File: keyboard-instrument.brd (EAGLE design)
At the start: 68.6 x 53.3 mm, 9 parts

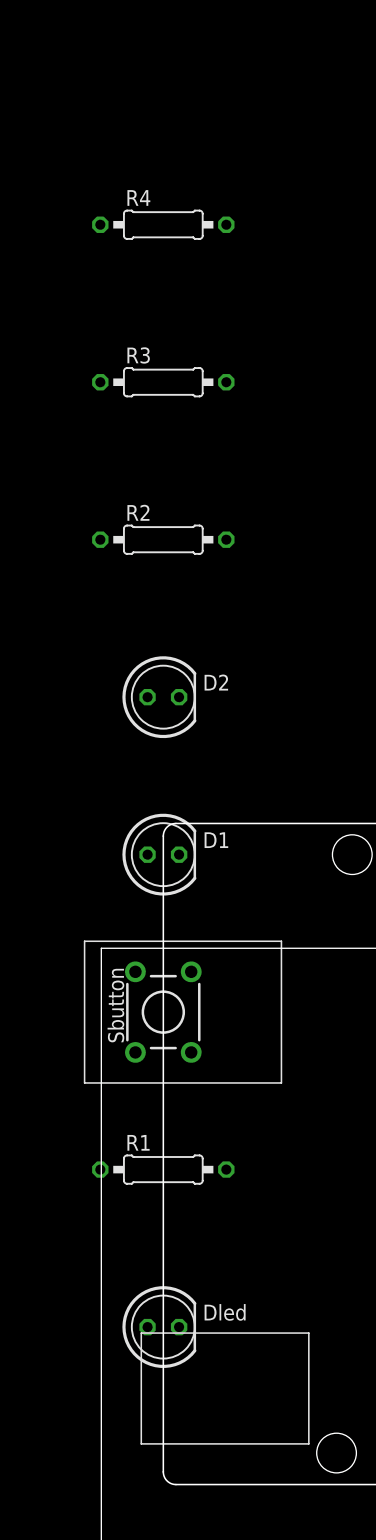
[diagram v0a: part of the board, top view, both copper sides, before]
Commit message: Added code and brd
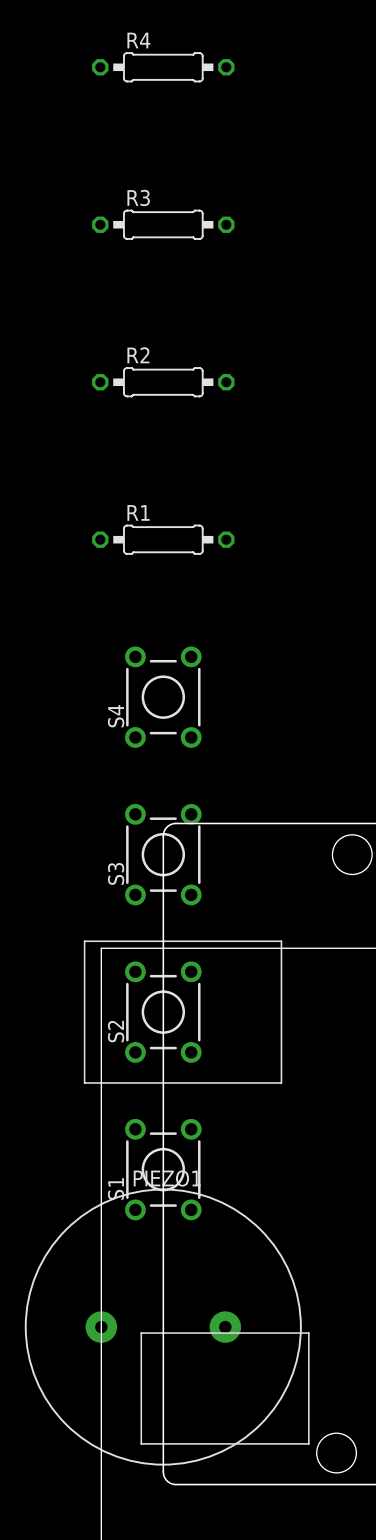
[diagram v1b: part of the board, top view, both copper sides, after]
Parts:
- removed D1, D2, Dled: (no value), AUTODESK_CIRCUITS_BREADBOARD:LED5MM
- added PIEZO1: (no value), AUTODESK_CIRCUITS_BREADBOARD:PIEZO-22MM
- added S1, S3, S4: (no value), AUTODESK_CIRCUITS_BREADBOARD:TL1105
- R1: value 1k‎Ω -> 220‎Ω
- R2, R4: value 1k‎Ω -> 10000‎Ω
- R3: value 1k‎Ω -> 1000000‎Ω
- moved R1 50.8 mm to (5.00, 86.3)
- moved R2 12.7 mm to (5.00, 99.0)
- moved R3 12.7 mm to (5.00, 111.7)
- moved R4 12.7 mm to (5.00, 124.4)
- renumbered Sbutton to S2, Uboard to U1
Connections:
- removed net N$5 (its old number): D2.K, R1.2
- removed net N$6 (its old number): D2.A, U1.5
- new net N$10: R2.1, S3.3
- new net N$11: S4.2
- new net N$12: S4.1
- new net N$13: R3.1, S4.3
- new net N$14: R4.1, S1.4, S2.4, S3.4, S4.4, U1.A0
- net N$1: now also PIEZO1.P$1, R1.2, R2.2, R3.2, R4.2, S1.3, U1.5V; no longer R1.1, R2.1, R3.1, R4.1
- net N$2: now also PIEZO1.P$2, U1.8; no longer S2.3, U1.5V
- net N$3: now also S1.2; no longer Dled.K, R4.2
- net N$4: now also S1.1; no longer Dled.A, U1.3
- net N$7: now also R1.1, S2.3; no longer D1.K, R3.2
- net N$8: now also S3.2; no longer D1.A, U1.4
- net N$9: now also S3.1; no longer R2.2, S2.4, U1.2
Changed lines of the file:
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@@
 </autorouter>
 <elements>
-<element value="" name="Uboard" library="AUTODESK_CIRCUITS_BREADBOARD" package="ARDUINO_UNO" x="5" y="10.08"></element><element value="" name="Dled" library="AUTODESK_CIRCUITS_BREADBOARD" package="LED5MM" x="5" y="22.78"></element><element value="1k‎Ω" name="R1" library="AUTODESK_CIRCUITS_BREADBOARD" package="0207/10" x="5" y="35.480000000000004"></element><element value="" name="Sbutton" library="AUTODESK_CIRCUITS_BREADBOARD" package="TL1105" x="5" y="48.18"></element><element value="" name="D1" library="AUTODESK_CIRCUITS_BREADBOARD" package="LED5MM" x="5" y="60.879999999999995"></element><element value="" name="D2" library="AUTODESK_CIRCUITS_BREADBOARD" package="LED5MM" x="5" y="73.58"></element><element value="1k‎Ω" name="R2" library="AUTODESK_CIRCUITS_BREADBOARD" package="0207/10" x="5" y="86.28"></element><element value="1k‎Ω" name="R3" library="AUTODESK_CIRCUITS_BREADBOARD" package="0207/10" x="5" y="98.98"></element><element value="1k‎Ω" name="R4" library="AUTODESK_CIRCUITS_BREADBOARD" package="0207/10" x="5" y="111.68"></element></elements>
+<element value="" name="U1" library="AUTODESK_CIRCUITS_BREADBOARD" package="ARDUINO_UNO" x="5" y="10.08"></element><element value="" name="PIEZO1" library="AUTODESK_CIRCUITS_BREADBOARD" package="PIEZO-22MM" x="5" y="22.78"></element><element value="" name="S1" library="AUTODESK_CIRCUITS_BREADBOARD" package="TL1105" x="5" y="35.480000000000004"></element><element value="" name="S2" library="AUTODESK_CIRCUITS_BREADBOARD" package="TL1105" x="5" y="48.18"></element><element value="" name="S3" library="AUTODESK_CIRCUITS_BREADBOARD" package="TL1105" x="5" y="60.879999999999995"></element><element value="" name="S4" library="AUTODESK_CIRCUITS_BREADBOARD" package="TL1105" x="5" y="73.58"></element><element value="220‎Ω" name="R1" library="AUTODESK_CIRCUITS_BREADBOARD" package="0207/10" x="5" y="86.28"></element><element value="10000‎Ω" name="R2" library="AUTODESK_CIRCUITS_BREADBOARD" package="0207/10" x="5" y="98.98"></element><element value="1000000‎Ω" name="R3" library="AUTODESK_CIRCUITS_BREADBOARD" package="0207/10" x="5" y="111.68"></element><element value="10000‎Ω" name="R4" library="AUTODESK_CIRCUITS_BREADBOARD" package="0207/10" x="5" y="124.38000000000001"></element></elements>
 <signals>
-<signal name="N$1"><contactref element="Uboard" pad="GND.."></contactref><contactref element="R2" pad="1"></contactref><wire x1="45.64" y1="12.620000000000001" x2="-0.08000000000000007" y2="86.28" width="0" layer="19" extent="1-1"></wire><contactref element="R1" pad="1"></contactref><wire x1="-0.08000000000000007" y1="86.28" x2="-0.08000000000000007" y2="35.480000000000004" width="0" layer="19" extent="1-1"></wire><contactref element="R3" pad="1"></contactref><wire x1="-0.08000000000000007" y1="35.480000000000004" x2="-0.08000000000000007" y2="98.98" width="0" layer="19" extent="1-1"></wire><contactref element="R4" pad="1"></contactref><wire x1="-0.08000000000000007" y1="98.98" x2="-0.08000000000000007" y2="111.68" width="0" layer="19" extent="1-1"></wire></signal><signal name="N$2"><contactref element="Uboard" pad="5V"></contactref><contactref element="Sbutton" pad="3"></contactref><wire x1="43.1" y1="12.620000000000001" x2="2.75" y2="44.93" width="0" layer="19" extent="1-1"></wire></signal><signal name="N$3"><contactref element="Dled" pad="K"></contactref><contactref element="R4" pad="2"></contactref><wire x1="6.27" y1="22.78" x2="10.08" y2="111.68" width="0" layer="19" extent="1-1"></wire></signal><signal name="N$4"><contactref element="Dled" pad="A"></contactref><contactref element="Uboard" pad="3"></contactref><wire x1="3.73" y1="22.78" x2="60.88" y2="60.879999999999995" width="0" layer="19" extent="1-1"></wire></signal><signal name="N$5"><contactref element="D2" pad="K"></contactref><contactref element="R1" pad="2"></contactref><wire x1="6.27" y1="73.58" x2="10.08" y2="35.480000000000004" width="0" layer="19" extent="1-1"></wire></signal><signal name="N$6"><contactref element="D2" pad="A"></contactref><contactref element="Uboard" pad="5"></contactref><wire x1="3.73" y1="73.58" x2="55.8" y2="60.879999999999995" width="0" layer="19" extent="1-1"></wire></signal><signal name="N$7"><contactref element="D1" pad="K"></contactref><contactref element="R3" pad="2"></contactref><wire x1="6.27" y1="60.879999999999995" x2="10.08" y2="98.98" width="0" layer="19" extent="1-1"></wire></signal><signal name="N$8"><contactref element="D1" pad="A"></contactref><contactref element="Uboard" pad="4"></contactref><wire x1="3.73" y1="60.879999999999995" x2="58.34" y2="60.879999999999995" width="0" layer="19" extent="1-1"></wire></signal><signal name="N$9"><contactref element="Sbutton" pad="4"></contactref><contactref element="Uboard" pad="2"></contactref><wire x1="7.25" y1="44.93" x2="63.42" y2="60.879999999999995" width="0" layer="19" extent="1-1"></wire><contactref element="R2" pad="2"></contactref><wire x1="63.42" y1="60.879999999999995" x2="10.08" y2="86.28" width="0" layer="19" extent="1-1"></wire></signal><signal name="N$10"><contactref element="Sbutton" pad="2"></contactref></signal><signal name="N$11"><contactref element="Sbutton" pad="1"></contactref></signal></signals>
+<signal name="N$1"><contactref element="U1" pad="GND.."></contactref><contactref element="R2" pad="2"></contactref><wire x1="45.64" y1="12.620000000000001" x2="10.08" y2="98.98" width="0" layer="19" extent="1-1"></wire><contactref element="R3" pad="2"></contactref><wire x1="10.08" y1="98.98" x2="10.08" y2="111.68" width="0" layer="19" extent="1-1"></wire><contactref element="R1" pad="2"></contactref><wire x1="10.08" y1="111.68" x2="10.08" y2="86.28" width="0" layer="19" extent="1-1"></wire><contactref element="S1" pad="3"></contactref><wire x1="10.08" y1="86.28" x2="2.75" y2="32.230000000000004" width="0" layer="19" extent="1-1"></wire><contactref element="U1" pad="5V"></contactref><wire x1="2.75" y1="32.230000000000004" x2="43.1" y2="12.620000000000001" width="0" layer="19" extent="1-1"></wire><contactref element="R4" pad="2"></contactref><wire x1="43.1" y1="12.620000000000001" x2="10.08" y2="124.38000000000001" width="0" layer="19" extent="1-1"></wire><contactref element="PIEZO1" pad="P$1"></contactref><wire x1="10.08" y1="124.38000000000001" x2="0" y2="22.78" width="0" layer="19" extent="1-1"></wire></signal><signal name="N$2"><contactref element="U1" pad="8"></contactref><contactref element="PIEZO1" pad="P$2"></contactref><wire x1="46.656" y1="60.879999999999995" x2="10" y2="22.78" width="0" layer="19" extent="1-1"></wire></signal><signal name="N$3"><contactref element="S1" pad="2"></contactref></signal><signal name="N$4"><contactref element="S1" pad="1"></contactref></signal><signal name="N$5"><contactref element="S2" pad="2"></contactref></signal><signal name="N$6"><contactref element="S2" pad="1"></contactref></signal><signal name="N$7"><contactref element="S2" pad="3"></contactref><contactref element="R1" pad="1"></contactref><wire x1="2.75" y1="44.93" x2="-0.08000000000000007" y2="86.28" width="0" layer="19" extent="1-1"></wire></signal><signal name="N$8"><contactref element="S3" pad="2"></contactref></signal><signal name="N$9"><contactref element="S3" pad="1"></contactref></signal><signal name="N$10"><contactref element="S3" pad="3"></contactref><contactref element="R2" pad="1"></contactref><wire x1="2.75" y1="57.629999999999995" x2="-0.08000000000000007" y2="98.98" width="0" layer="19" extent="1-1"></wire></signal><signal name="N$11"><contactref element="S4" pad="2"></contactref></signal><signal name="N$12"><contactref element="S4" pad="1"></contactref></signal><signal name="N$13"><contactref element="S4" pad="3"></contactref><contactref element="R3" pad="1"></contactref><wire x1="2.75" y1="70.33" x2="-0.08000000000000007" y2="111.68" width="0" layer="19" extent="1-1"></wire></signal><signal name="N$14"><contactref element="R4" pad="1"></contactref><contactref element="S1" pad="4"></contactref><wire x1="-0.08000000000000007" y1="124.38000000000001" x2="7.25" y2="32.230000000000004" width="0" layer="19" extent="1-1"></wire><contactref element="S2" pad="4"></contactref><wire x1="7.25" y1="32.230000000000004" x2="7.25" y2="44.93" width="0" layer="19" extent="1-1"></wire><contactref element="S3" pad="4"></contactref><wire x1="7.25" y1="44.93" x2="7.25" y2="57.629999999999995" width="0" layer="19" extent="1-1"></wire><contactref element="S4" pad="4"></contactref><wire x1="7.25" y1="57.629999999999995" x2="7.25" y2="70.33" width="0" layer="19" extent="1-1"></wire><contactref element="U1" pad="A0"></contactref><wire x1="7.25" y1="70.33" x2="55.8" y2="12.620000000000001" width="0" layer="19" extent="1-1"></wire></signal></signals>
 </board>
 </drawing>
